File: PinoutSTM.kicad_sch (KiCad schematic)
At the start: 21 parts, among them IC1 STM32H7B0RBT6, J4 1761681-3, J6 Header male 1x05, Q1 50V, SW1 Button Switch SPST-No, Y1 CC4V-T1A-32.768kHz-6pF-20PPM-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

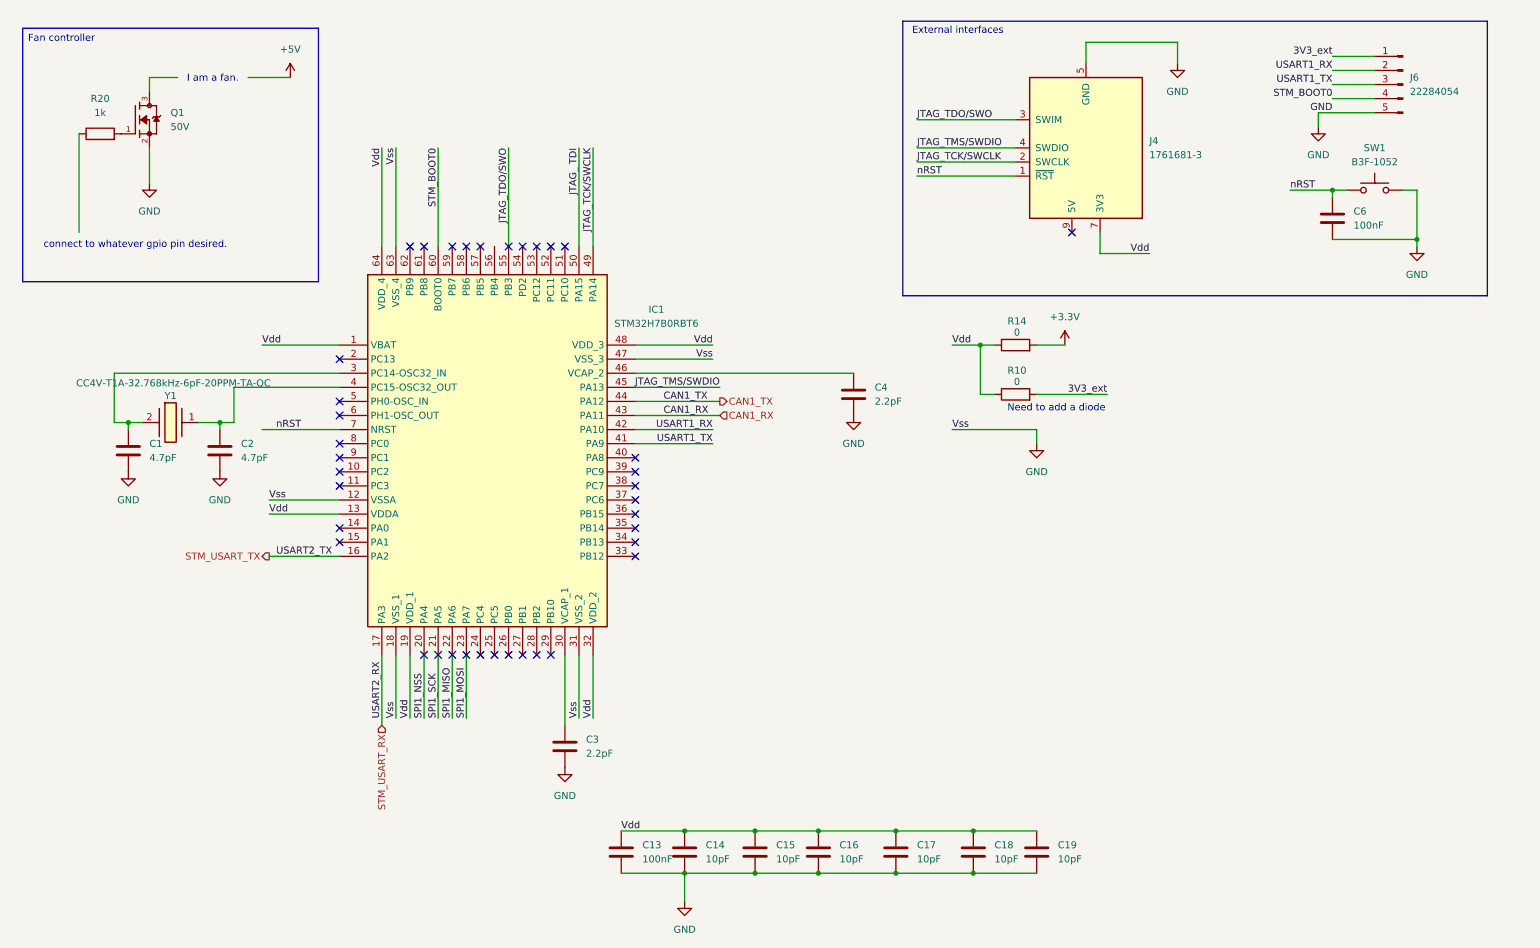
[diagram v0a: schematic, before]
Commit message: Added Power logic finally. (plus some comments on further improvements)
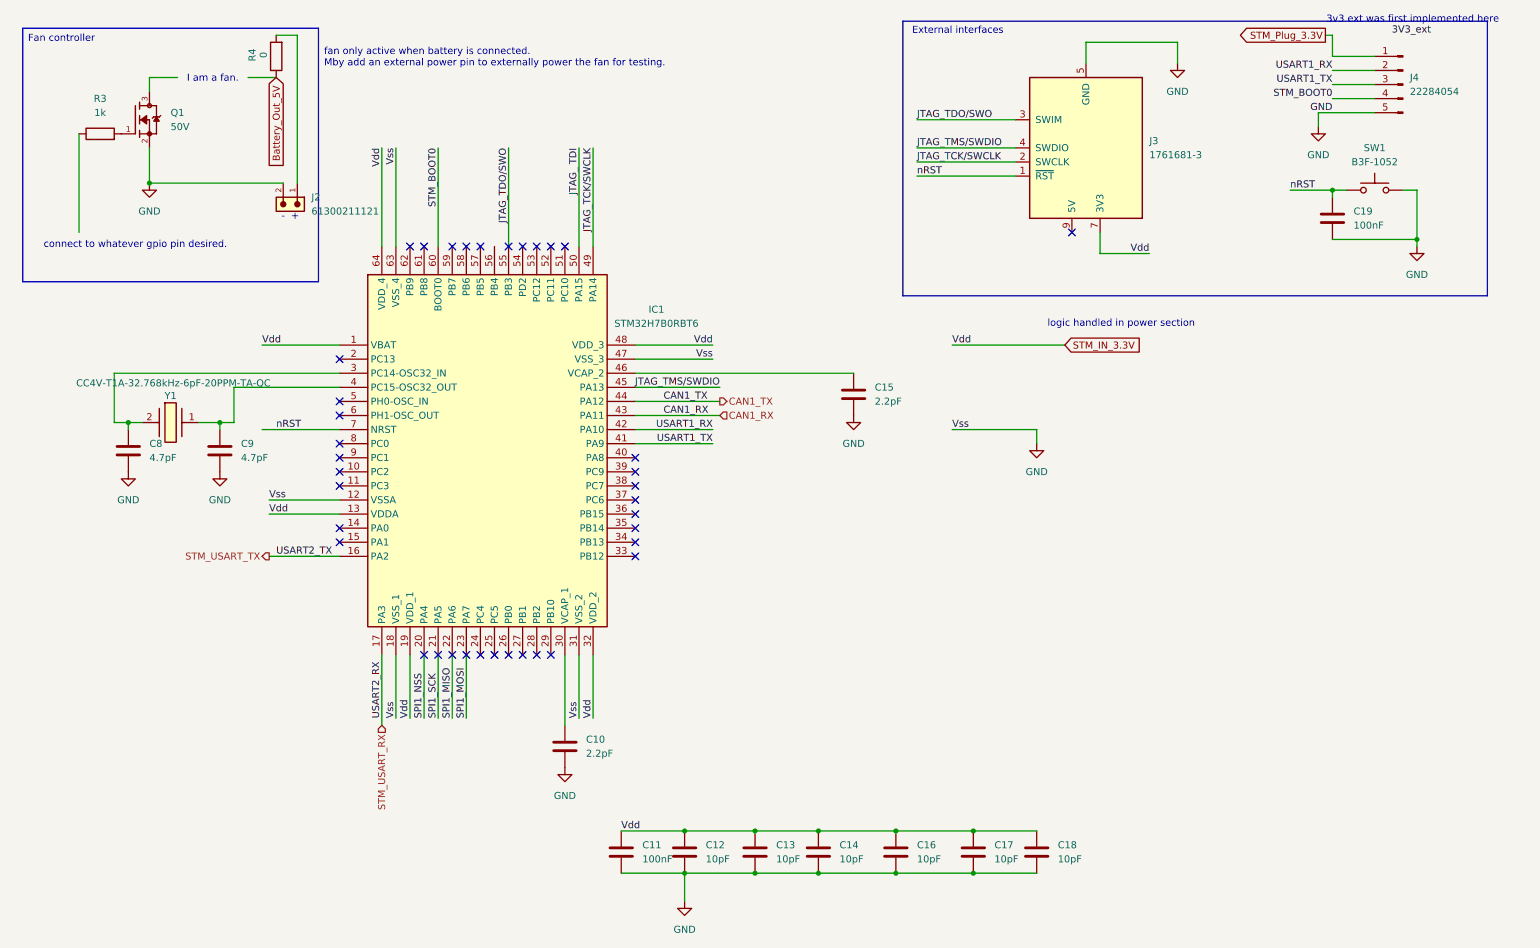
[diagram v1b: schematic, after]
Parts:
- removed R10, R14: 0, Resistor_SMD:R_0603_1608Metric, symbol #dzdb:g_res/R-0-0603
- added J2: 61300211121, dz_con:Wurth_Con_61300211121, symbol #dzdb:s_con/WURT-61300211121
- added R4: 0, Resistor_SMD:R_0603_1608Metric, symbol #dzdb:g_res/R-0-0603
- renumbered C3 to C10, C13 to C11, C14 to C12, C15 to C13, C16 to C14, C4 to C15, C17 to C16, C18 to C17, C19 to C18, C6 to C19, C1 to C8, C2 to C9, J4 to J3, J6 to J4, R20 to R3
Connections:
- net 3V3_ext: no longer J4.1 (Pin_1)
- net GND: now also J2.2
- net Vdd renamed STM_IN_3.3V
- new net: J2.1, R4.2
- new net Battery_Out_5V: R4.1
- new net STM_Plug_3.3V: J4.1 (Pin_1)
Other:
- note added: "- +"
- note added: "3v3 ext was first implemented here"
- note added: "fan only active when battery is connected. Mby add an external power pin to externally power the fan for testing."
- note added: "logic handled in power section"
- note removed: "Need to add a diode"
